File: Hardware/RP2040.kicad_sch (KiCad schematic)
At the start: 1 part, among them U1 RP2040

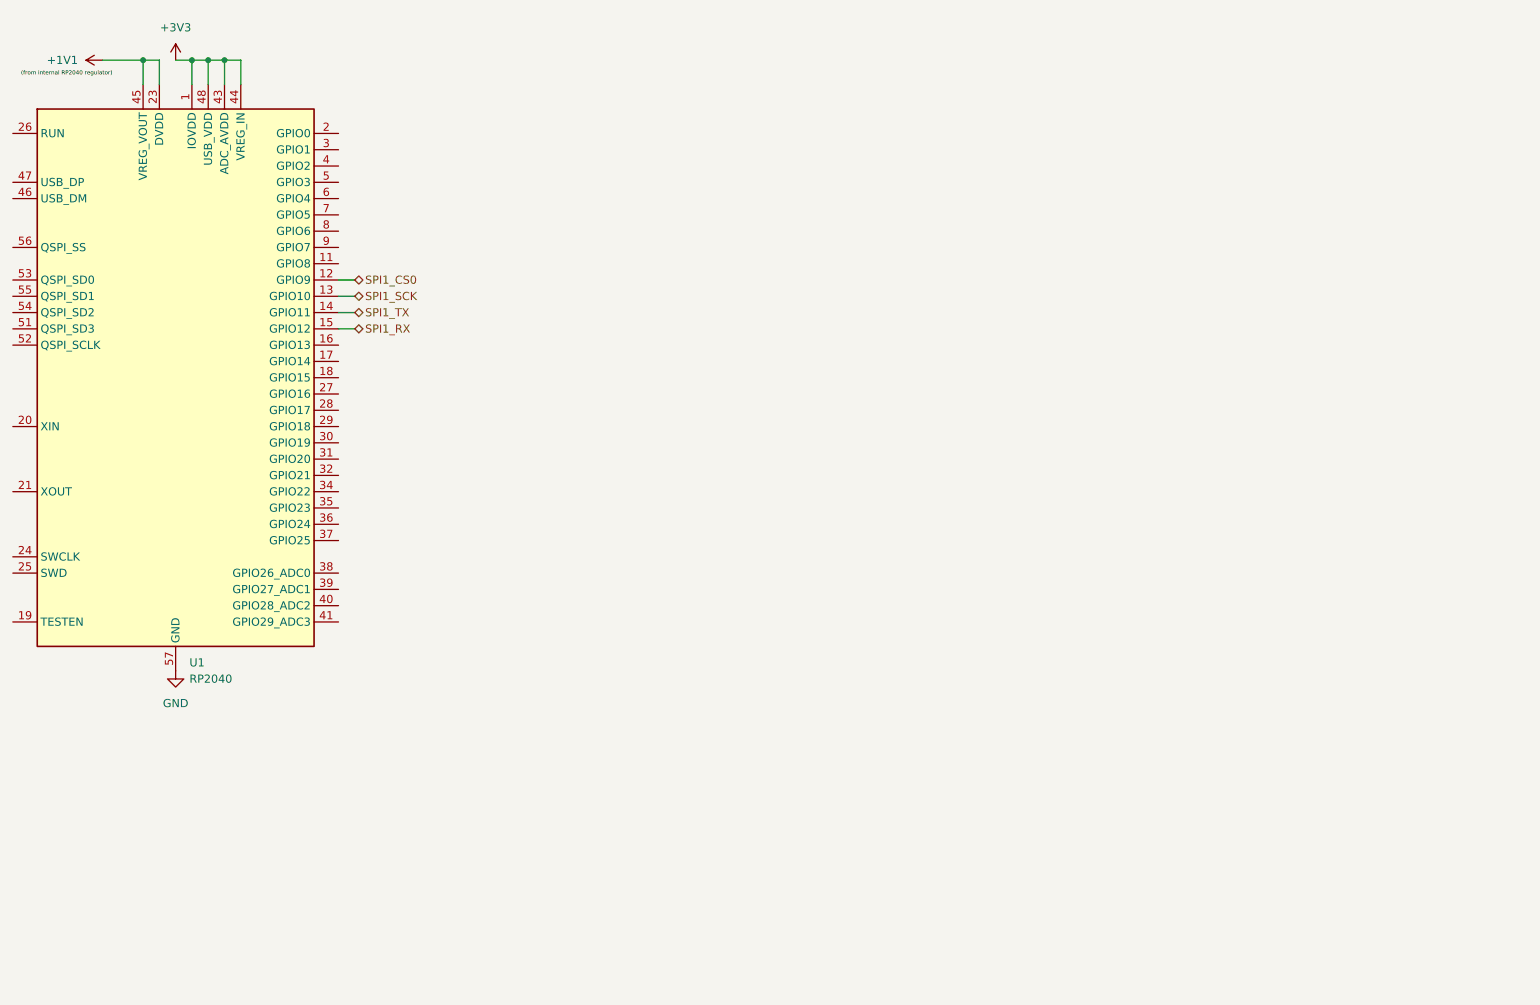
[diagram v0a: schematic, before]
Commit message: RP2040 Schematic
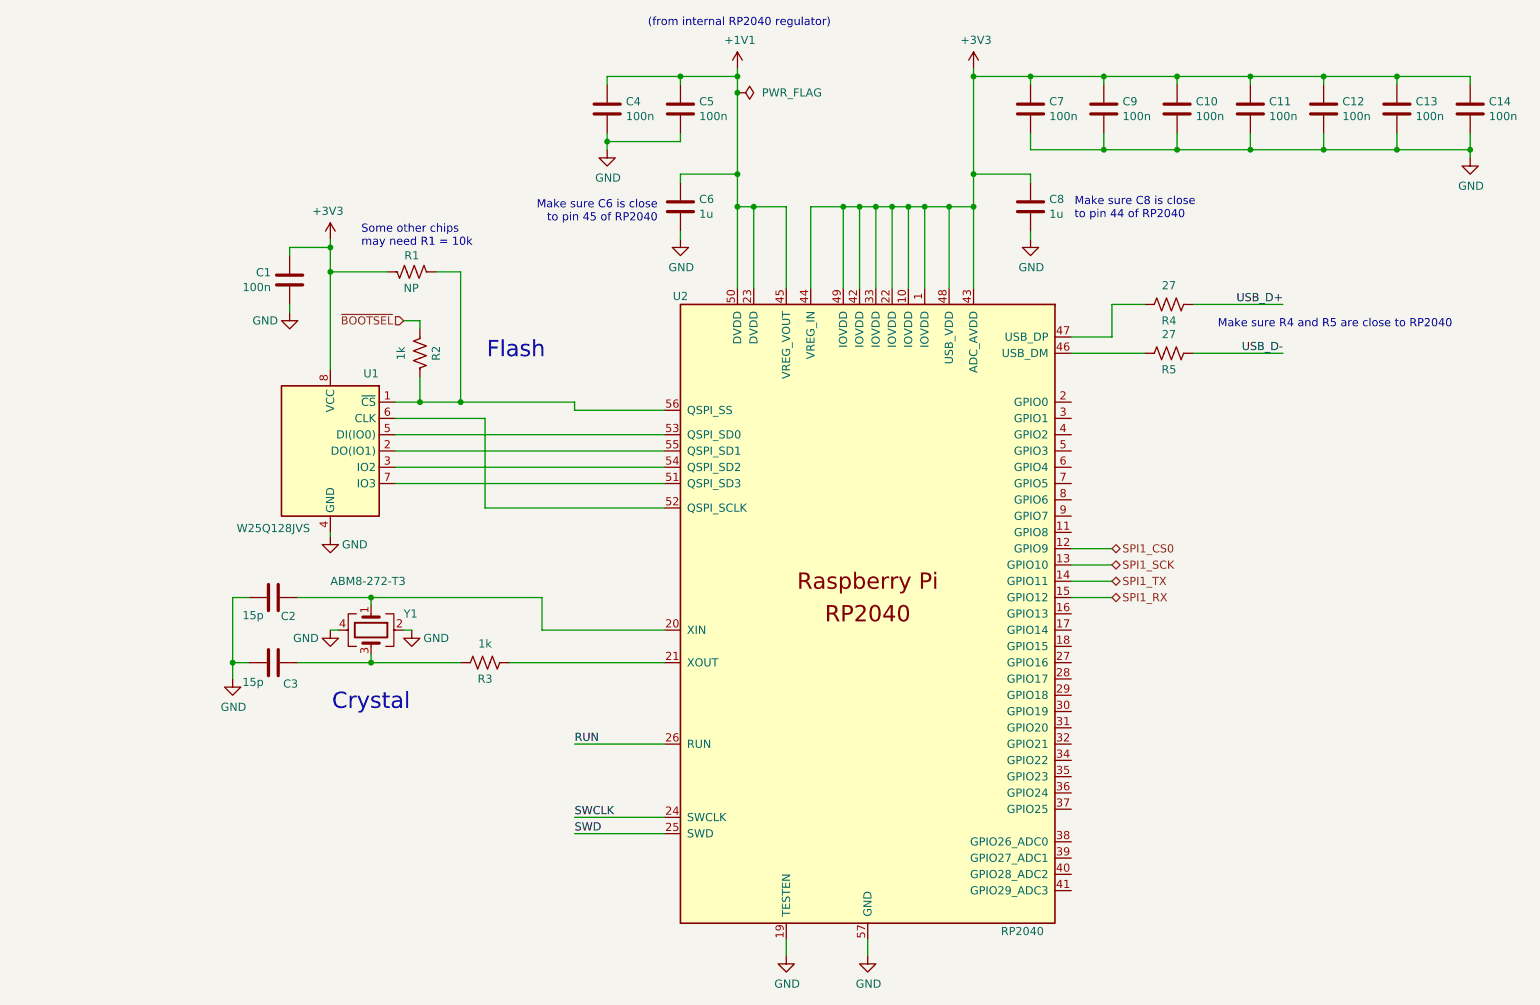
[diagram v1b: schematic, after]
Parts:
- removed U1: RP2040, Package_DFN_QFN:QFN-56-1EP_7x7mm_P0.4mm_EP3.2x3.2mm, symbol MCU_RaspberryPi:RP2040
- added C1, C10, C11, C12, C13, C14, C4, C5, C7, C9: 100n, Capacitor_SMD:C_0402_1005Metric, symbol Device:C
- added C2, C3: 15p, Capacitor_SMD:C_0402_1005Metric, symbol Device:C
- added C6, C8: 1u, Capacitor_SMD:C_0402_1005Metric, symbol Device:C
- added R1: NP, Resistor_SMD:R_0402_1005Metric, symbol Device:R_US
- added R2, R3: 1k, Resistor_SMD:R_0402_1005Metric, symbol Device:R_US
- added R4, R5: 27, Resistor_SMD:R_0402_1005Metric, symbol Device:R_US
- added U1: W25Q128JVS, Package_SO:SOIC-8_5.23x5.23mm_P1.27mm, symbol Memory_Flash:W25Q128JVS
- added U2: RP2040, RP2040:RP2040-QFN-56, symbol RP2040:RP2040
- added Y1: ABM8-272-T3, Crystal:Crystal_SMD_3225-4Pin_3.2x2.5mm, symbol Device:Crystal_GND24
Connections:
- net +1V1: now also C4.1, C5.1, C6.1, U2.23 (DVDD), U2.45 (VREG_VOUT), U2.50 (DVDD)
- net +3V3: now also C1.1, C10.1, C11.1, C12.1, C13.1, C14.1, C7.1, C8.1, C9.1, R1.2, U1.8 (VCC), U2.1 (IOVDD), U2.10 (IOVDD), U2.22 (IOVDD), U2.33 (IOVDD), U2.42 (IOVDD), U2.43 (ADC_AVDD), U2.44 (VREG_IN), U2.48 (USB_VDD), U2.49 (IOVDD)
- net GND: now also C1.2, C10.2, C11.2, C12.2, C13.2, C14.2, C2.2, C3.2, C4.2, C5.2, C6.2, C7.2, C8.2, C9.2, U1.4 (GND), U2.19 (TESTEN), U2.57 (GND), Y1.2, Y1.4
- net SPI1_CS0: now also U2.12 (GPIO9)
- net SPI1_RX: now also U2.15 (GPIO12)
- net SPI1_SCK: now also U2.13 (GPIO10)
- net SPI1_TX: now also U2.14 (GPIO11)
- new net: C2.1, U2.20 (XIN), Y1.1
- new net: R3.1, U2.21 (XOUT)
- new net: R5.2, U2.46 (USB_DM)
- new net: R4.2, U2.47 (USB_DP)
- new net: U1.7 (IO3), U2.51 (QSPI_SD3)
- new net: U1.6 (CLK), U2.52 (QSPI_SCLK)
- new net: U1.5 (DI(IO0)), U2.53 (QSPI_SD0)
- new net: U1.3 (IO2), U2.54 (QSPI_SD2)
- new net: U1.2 (DO(IO1)), U2.55 (QSPI_SD1)
- new net: R1.1, R2.1, U1.1 (~{CS}), U2.56 (QSPI_SS)
- new net: C3.1, R3.2, Y1.3
- new net RUN: U2.26 (RUN)
- new net SWCLK: U2.24 (SWCLK)
- new net SWD: U2.25 (SWD)
- new net USB_D+: R4.1
- new net USB_D-: R5.1
- new net ~{BOOTSEL}: R2.2
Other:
- note added: "(from internal RP2040 regulator)"
- note added: "Crystal"
- note added: "Flash"
- note added: "Make sure C6 is close to pin 45 of RP2040"
- note added: "Make sure C8 is close to pin 44 of RP2040"
- note added: "Make sure R4 and R5 are close to RP2040"
- note added: "Some other chips may need R1 = 10k"
